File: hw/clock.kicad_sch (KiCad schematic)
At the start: 1 part, among them X1 1MHz

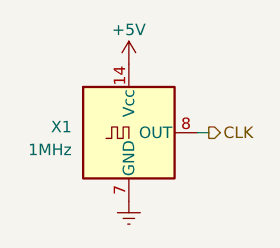
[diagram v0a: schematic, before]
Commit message: add hw design for veraduino
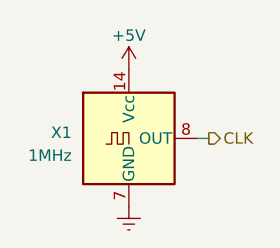
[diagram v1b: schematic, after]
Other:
- moved on the sheet: X1
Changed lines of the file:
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@@
 (kicad_sch (version 20230121) (generator eeschema)
   (paper "A4")
-  (wire (pts (xy 50.8 36.195) (xy 49.53 36.195))
+  (wire (pts (xy 50.8 36.83) (xy 49.53 36.83))
     (stroke (width 0) (type default))
   )
-  (hierarchical_label "CLK" (shape output) (at 50.8 36.195 0) (fields_autoplaced)
+  (hierarchical_label "CLK" (shape output) (at 50.8 36.83 0) (fields_autoplaced)
     (effects (font (size 1.27 1.27)) (justify left))
   )
-  (symbol (lib_id "power:VCC") (at 41.91 28.575 0) (unit 1)
+  (symbol (lib_id "power:VCC") (at 41.91 29.21 0) (unit 1)
     (in_bom yes) (on_board yes) (dnp no) (fields_autoplaced)
-    (property "Reference" "#PWR01" (at 41.91 32.385 0)
+    (property "Reference" "#PWR01" (at 41.91 33.02 0)
       (effects (font (size 1.27 1.27)) hide)
     )
-    (property "Value" "+5V" (at 41.91 24.765 0)
+    (property "Value" "+5V" (at 41.91 25.4 0)
       (effects (font (size 1.27 1.27)))
     )
-    (property "Footprint" "" (at 41.91 28.575 0)
+    (property "Footprint" "" (at 41.91 29.21 0)
       (effects (font (size 1.27 1.27)) hide)
     )
-    (property "Datasheet" "" (at 41.91 28.575 0)
+    (property "Datasheet" "" (at 41.91 29.21 0)
       (effects (font (size 1.27 1.27)) hide)
     )
@@
     )
   )
-  (symbol (lib_id "Oscillator:ACO-xxxMHz") (at 41.91 36.195 0) (unit 1)
+  (symbol (lib_id "Oscillator:ACO-xxxMHz") (at 41.91 36.83 0) (unit 1)
     (in_bom yes) (on_board yes) (dnp no) (fields_autoplaced)
-    (property "Reference" "X1" (at 35.56 35.56 0)
+    (property "Reference" "X1" (at 35.56 36.195 0)
       (effects (font (size 1.27 1.27)) (justify right))
     )
-    (property "Value" "1MHz" (at 35.56 38.1 0)
+    (property "Value" "1MHz" (at 35.56 38.735 0)
       (effects (font (size 1.27 1.27)) (justify right))
     )
-    (property "Footprint" "Oscillator:Oscillator_DIP-14" (at 53.34 45.085 0)
+    (property "Footprint" "Oscillator:Oscillator_DIP-14" (at 53.34 45.72 0)
       (effects (font (size 1.27 1.27)) hide)
     )
-    (property "Datasheet" "http://www.conwin.com/datasheets/cx/cx030.pdf" (at 39.37 36.195 0)
+    (property "Datasheet" "http://www.conwin.com/datasheets/cx/cx030.pdf" (at 39.37 36.83 0)
       (effects (font (size 1.27 1.27)) hide)
     )
@@
     )
   )
-  (symbol (lib_id "power:Earth") (at 41.91 43.815 0) (unit 1)
+  (symbol (lib_id "power:Earth") (at 41.91 44.45 0) (unit 1)
     (in_bom yes) (on_board yes) (dnp no) (fields_autoplaced)
-    (property "Reference" "#PWR04" (at 41.91 50.165 0)
+    (property "Reference" "#PWR04" (at 41.91 50.8 0)
       (effects (font (size 1.27 1.27)) hide)
     )
-    (property "Value" "Earth" (at 41.91 47.625 0)
+    (property "Value" "Earth" (at 41.91 48.26 0)
       (effects (font (size 1.27 1.27)) hide)
     )
-    (property "Footprint" "" (at 41.91 43.815 0)
+    (property "Footprint" "" (at 41.91 44.45 0)
       (effects (font (size 1.27 1.27)) hide)
     )
-    (property "Datasheet" "~" (at 41.91 43.815 0)
+    (property "Datasheet" "~" (at 41.91 44.45 0)
       (effects (font (size 1.27 1.27)) hide)
     )
